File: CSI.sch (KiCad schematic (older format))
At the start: 14 parts

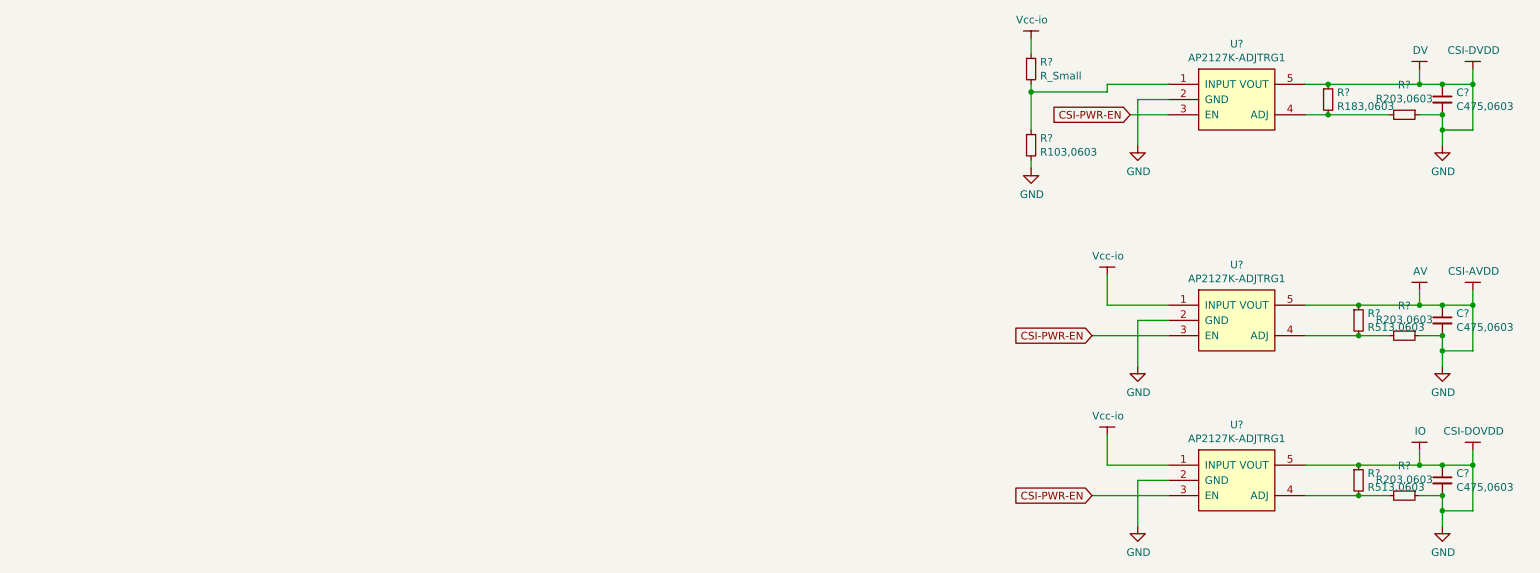
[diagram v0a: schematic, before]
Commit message: update CSI,
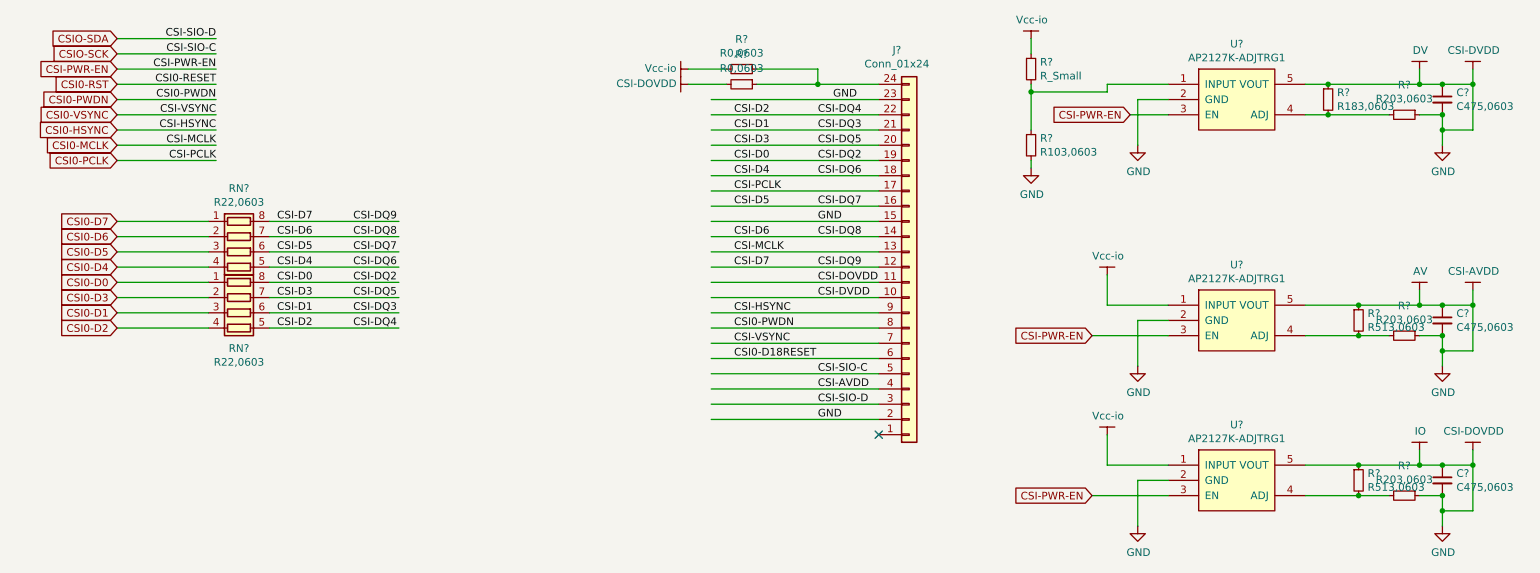
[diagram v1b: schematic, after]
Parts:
- added J?: Conn_01x24, symbol Connector_Generic:Conn_01x24
- added R? (x2): R0,0603, Resistor_SMD:R_0603_1608Metric_Pad1.05x0.95mm_HandSolder, symbol taobao-r:R0,0603
- added RN? (x2): R22,0603, symbol Device:R_Pack04
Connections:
- net labels added: CSI-D0, CSI-D1, CSI-D2, CSI-D3, CSI-D4, CSI-D5, CSI-D6, CSI-D7, CSI-DQ2, CSI-DQ3, CSI-DQ4, CSI-DQ5, CSI-DQ6, CSI-DQ7, CSI-DQ8, CSI-DQ9, CSI-HSYNC, CSI-MCLK, CSI-PCLK, CSI-SIO-C, CSI-SIO-D, CSI-VSYNC, CSI0-D0, CSI0-D1, CSI0-D18RESET, CSI0-D2, CSI0-D3, CSI0-D4, CSI0-D5, CSI0-D6, CSI0-D7, CSI0-HSYNC, CSI0-MCLK, CSI0-PCLK, CSI0-PWDN, CSI0-RESET, CSI0-RST, CSI0-VSYNC, CSIO-SCK, CSIO-SDA
- wire segments 59 -> 112
- no-connect marks 0 -> 1
